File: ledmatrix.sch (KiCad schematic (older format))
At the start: 70 parts, among them U2 sled1735

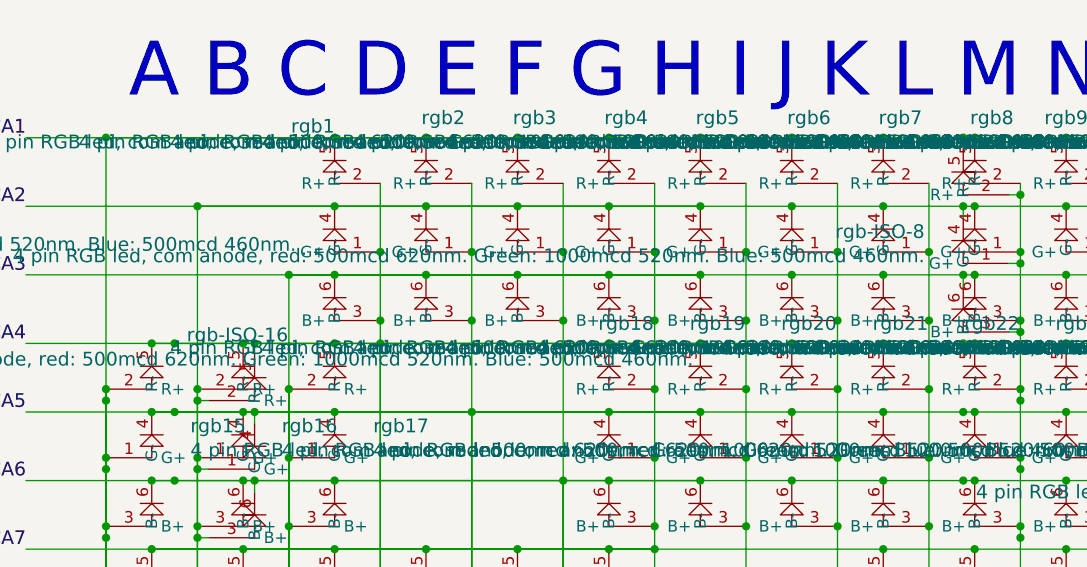
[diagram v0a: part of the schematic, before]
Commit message: pre align
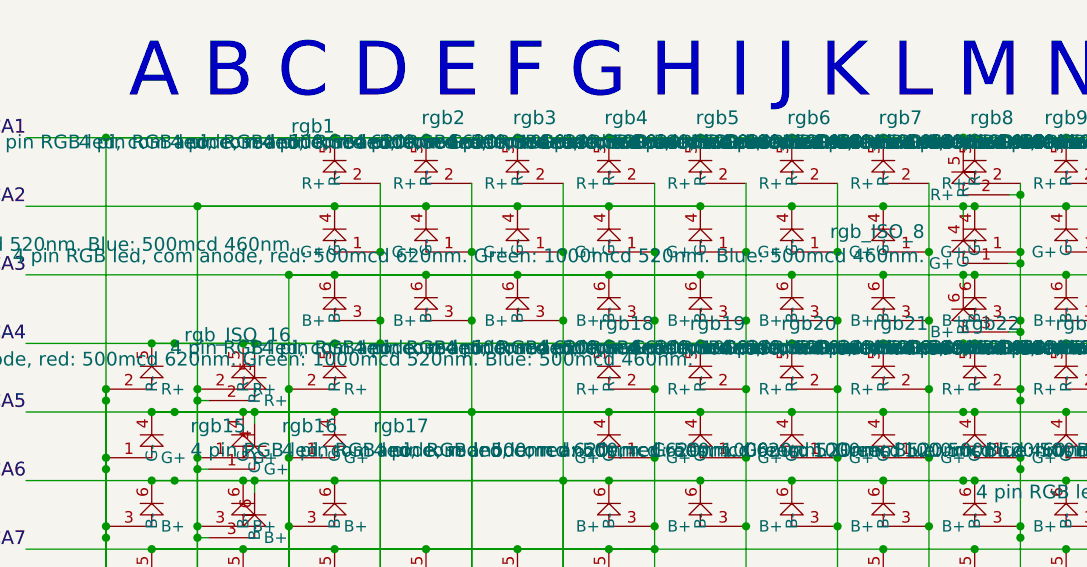
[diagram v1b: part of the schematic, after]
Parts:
- renumbered rgb-ISO-16 to rgb_ISO_16, rgb-ISO-8 to rgb_ISO_8
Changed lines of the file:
@@
 EESchema Schematic File Version 3
 LIBS:raise-right-asym-cache
-LIBS:power
-LIBS:74xx
 EELAYER 26 0
 EELAYER END
@@
 $EndComp
 $Comp
-L rgbled rgb-ISO-8
+L rgbled rgb_ISO_8
 U 1 1 5AE302CF
 P 5100 1550
-F 0 "rgb-ISO-8" H 4931 1689 60  0000 R CNN
+F 0 "rgb_ISO_8" H 4931 1689 60  0000 R CNN
 F 1 "4 pin RGB led, com anode, red: 500mcd 620nm. Green: 1000mcd 520nm. Blue: 500mcd 460nm." H 4931 1583 60  0000 R CNN
 F 2 "raise_fp:3528-4p-rev" H 5100 1550 60  0001 C CNN
@@
 Connection ~ 1350 2750
 $Comp
-L rgbled rgb-ISO-16
+L rgbled rgb_ISO_16
 U 1 1 5AE31270
 P 2000 2450
-F 0 "rgb-ISO-16" H 2075 3037 60  0000 C CNN
+F 0 "rgb_ISO_16" H 2075 3037 60  0000 C CNN
 F 1 "4 pin RGB led, com anode, red: 500mcd 620nm. Green: 1000mcd 520nm. Blue: 500mcd 460nm." H 2075 2931 60  0000 C CNN
 F 2 "raise_fp:3528-4p-rev" H 2000 2450 60  0001 C CNN
